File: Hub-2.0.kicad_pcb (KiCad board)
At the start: 2 copper layers, 120 x 78 mm, 9 parts, among them CN1 6437288-3, CN4 DT15-12PA, CN5 DT15-12PA, CN6 DT15-12PA, J3-PCB1 5569-06A2, U1 YQ506-S-112 DM

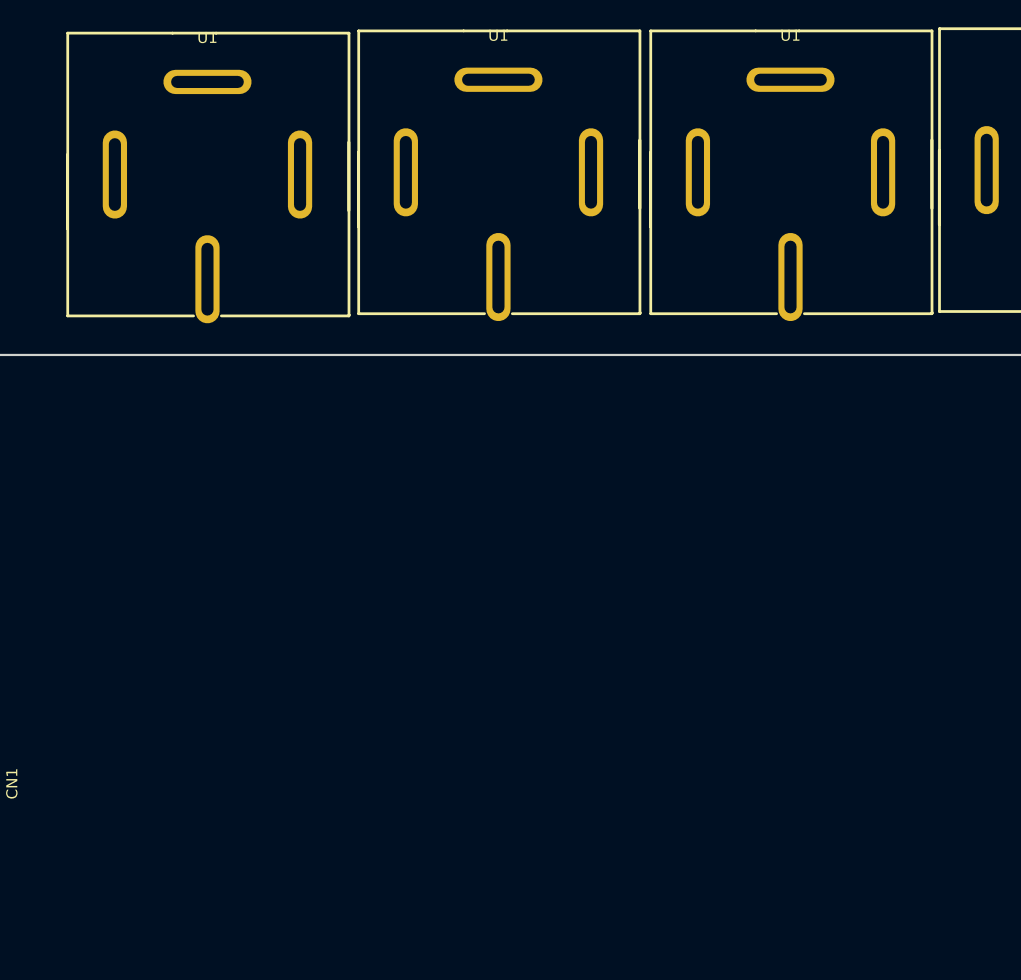
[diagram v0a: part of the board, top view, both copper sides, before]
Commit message: Autosave
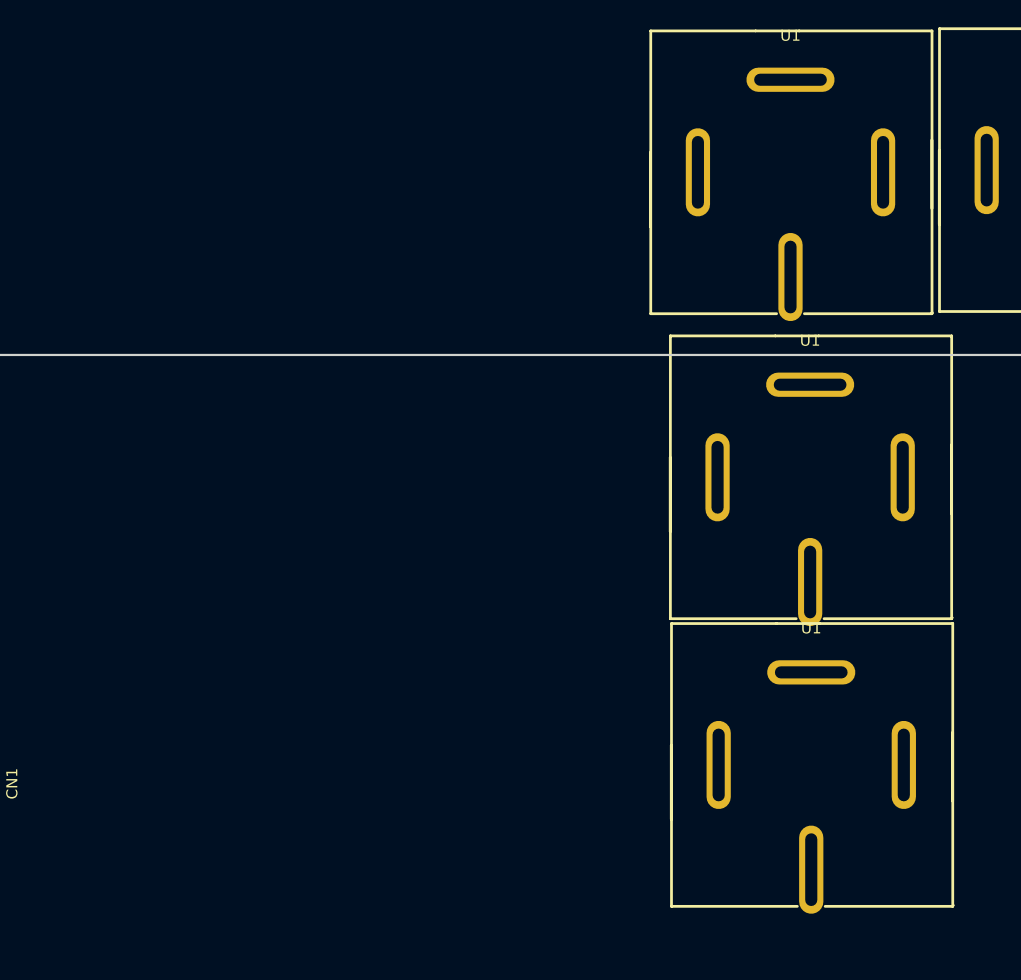
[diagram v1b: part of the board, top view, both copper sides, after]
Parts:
- moved U1 61.2 mm to (143.6, 40.5)
- moved U1 60.8 mm to (143.7, 66.5)
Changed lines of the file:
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@@
 	(footprint "EasyEDA:RELAY-TH_YQ506-S-112DM"
 		(layer "F.Cu")
-		(at 115.317502 12.7775)
+		(at 143.7 66.55)
 		(property "Reference" "U1"
 			(at 0 -12.95 0)
@@
 	(footprint "EasyEDA:RELAY-TH_YQ506-S-112DM"
 		(layer "F.Cu")
-		(at 88.9175 12.9775)
+		(at 143.6 40.45)
 		(property "Reference" "U1"
 			(at 0 -12.95 0)

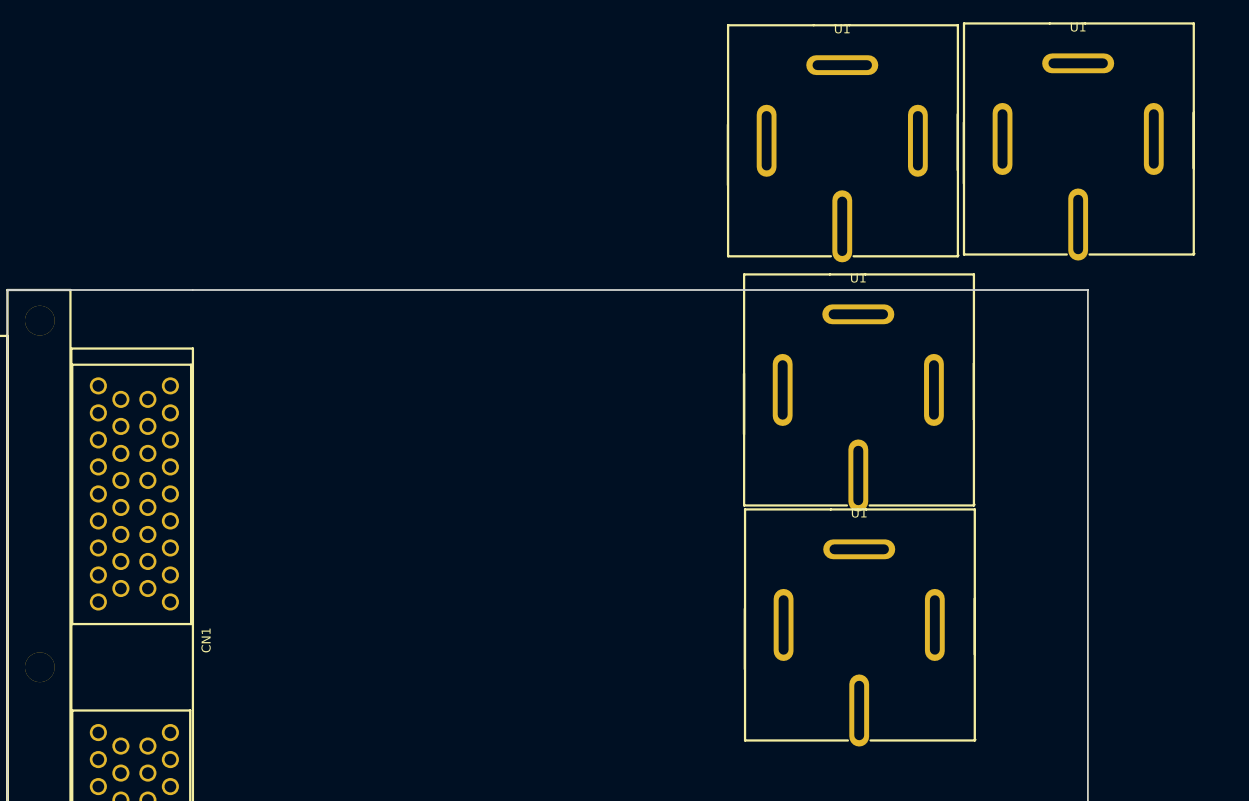
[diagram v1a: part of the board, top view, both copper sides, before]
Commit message: Autosave
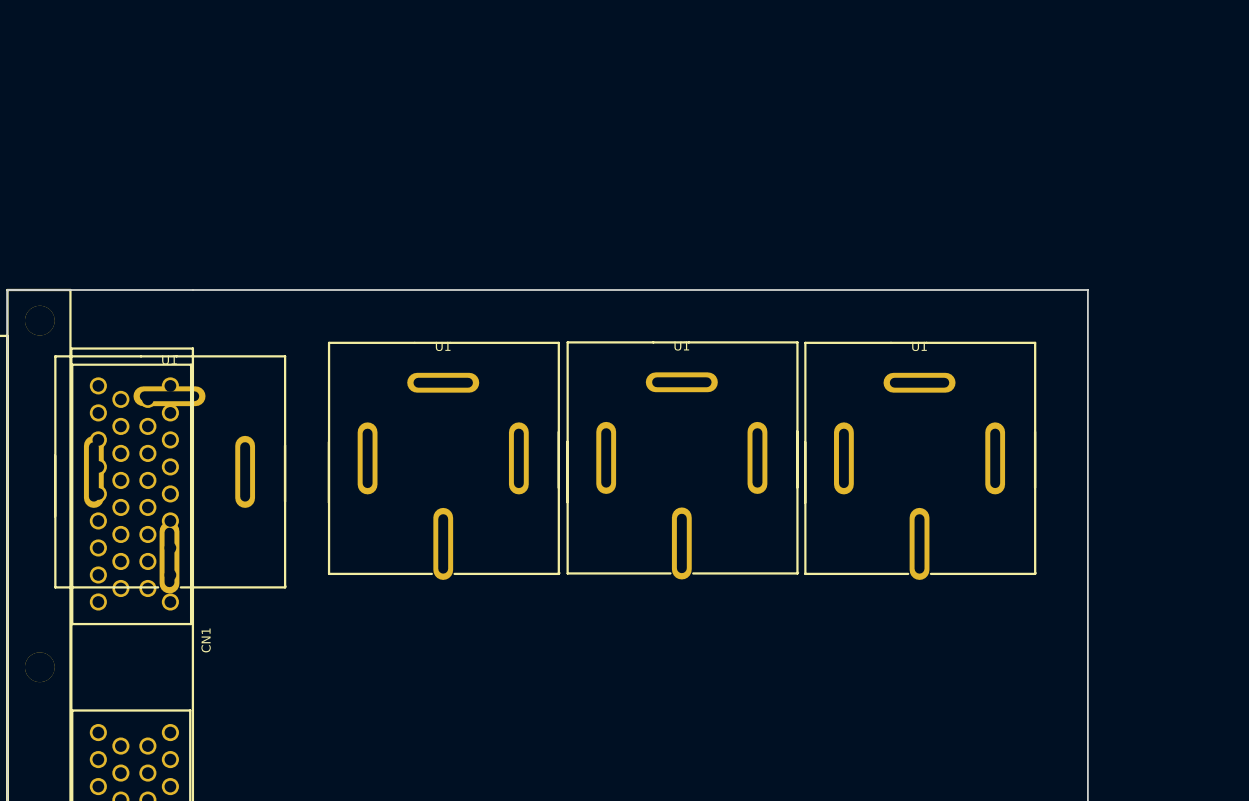
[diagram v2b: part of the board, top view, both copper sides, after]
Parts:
- moved U1 107.5 mm to (67.1, 49.5)
- moved U1 56.6 mm to (97.5, 48.0)
- moved U1 27.1 mm to (124.0, 48.0)
- moved U1 10.2 mm to (150.4, 48.0)
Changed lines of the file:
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@@
 	(footprint "EasyEDA:RELAY-TH_YQ506-S-112DM"
 		(layer "F.Cu")
-		(at 143.7 66.55)
+		(at 124 48)
 		(property "Reference" "U1"
 			(at 0 -12.95 0)
@@
 	(footprint "EasyEDA:RELAY-TH_YQ506-S-112DM"
 		(layer "F.Cu")
-		(at 143.6 40.45)
+		(at 150.4 48.05)
 		(property "Reference" "U1"
 			(at 0 -12.95 0)
@@
 	(footprint "EasyEDA:RELAY-TH_YQ506-S-112DM"
 		(layer "F.Cu")
-		(at 141.817501 12.7775)
+		(at 97.5 48.05)
 		(property "Reference" "U1"
 			(at 0 -12.95 0)
@@
 	(footprint "EasyEDA:RELAY-TH_YQ506-S-112DM"
 		(layer "F.Cu")
-		(at 168.0175 12.5775)
+		(at 67.1 49.55)
 		(property "Reference" "U1"
 			(at 0 -12.95 0)

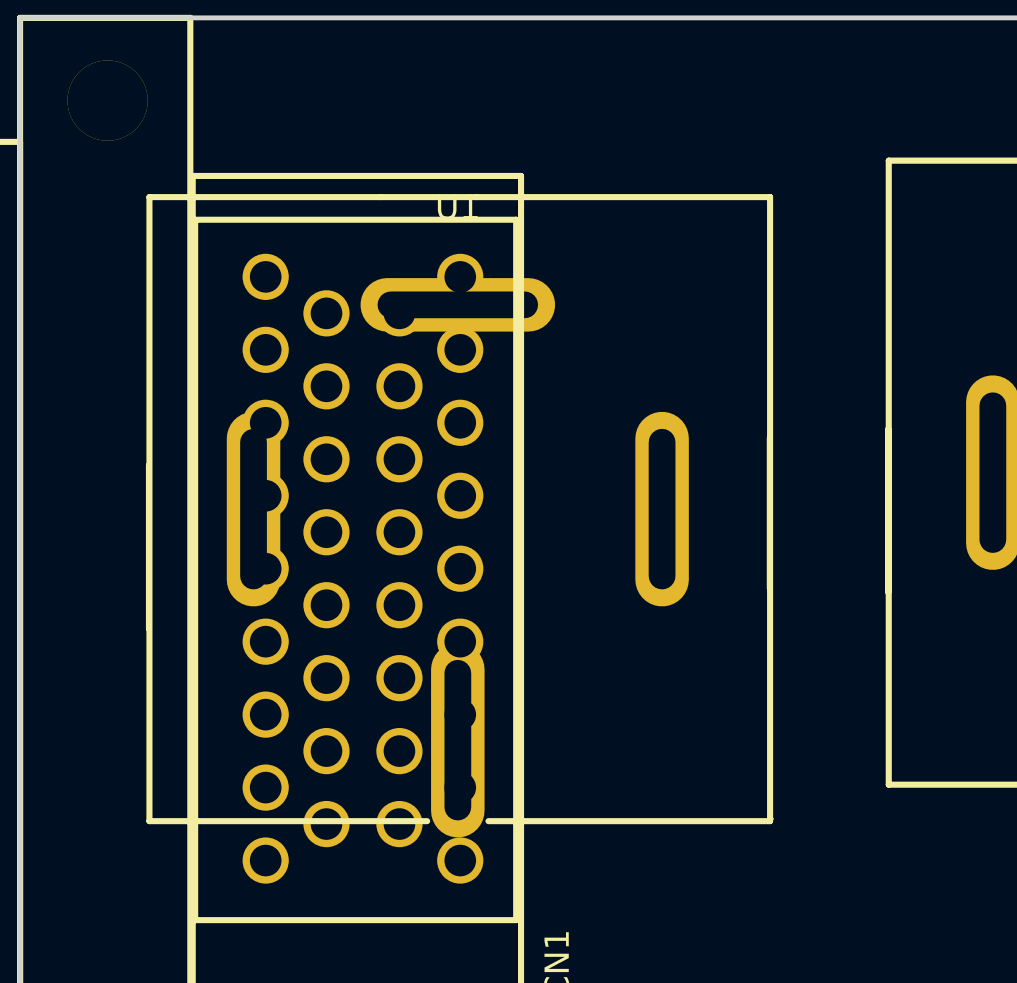
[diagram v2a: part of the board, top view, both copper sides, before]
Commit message: Autosave
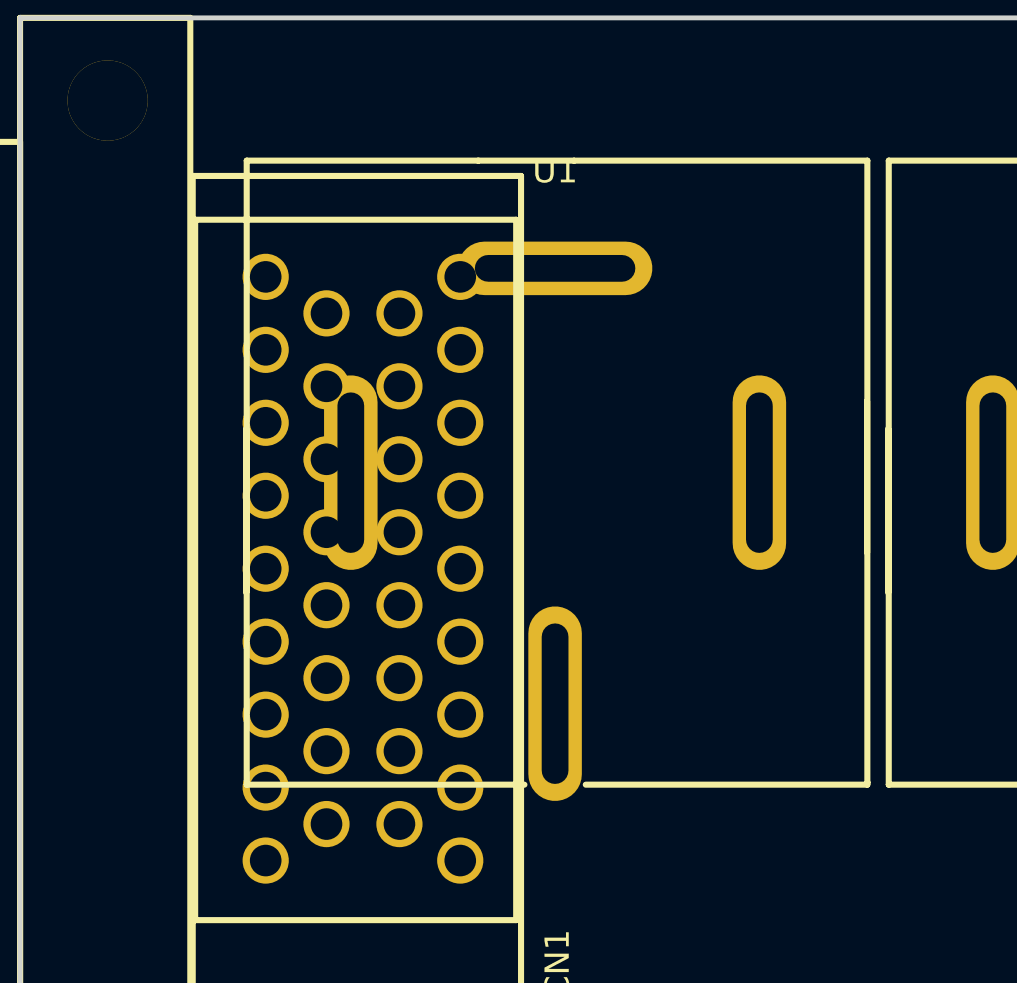
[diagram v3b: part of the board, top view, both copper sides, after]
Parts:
- moved U1 4.27 mm to (71.1, 48.0)
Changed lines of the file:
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@@
 	(footprint "EasyEDA:RELAY-TH_YQ506-S-112DM"
 		(layer "F.Cu")
-		(at 67.1 49.55)
+		(at 71.1 48.05)
 		(property "Reference" "U1"
 			(at 0 -12.95 0)

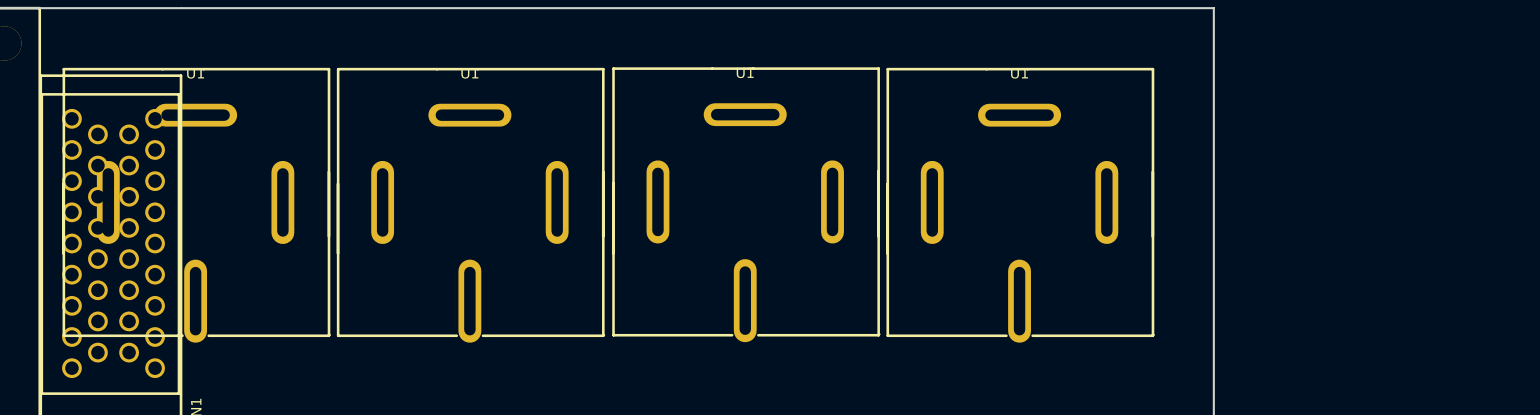
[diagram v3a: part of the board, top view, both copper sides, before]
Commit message: Autosave
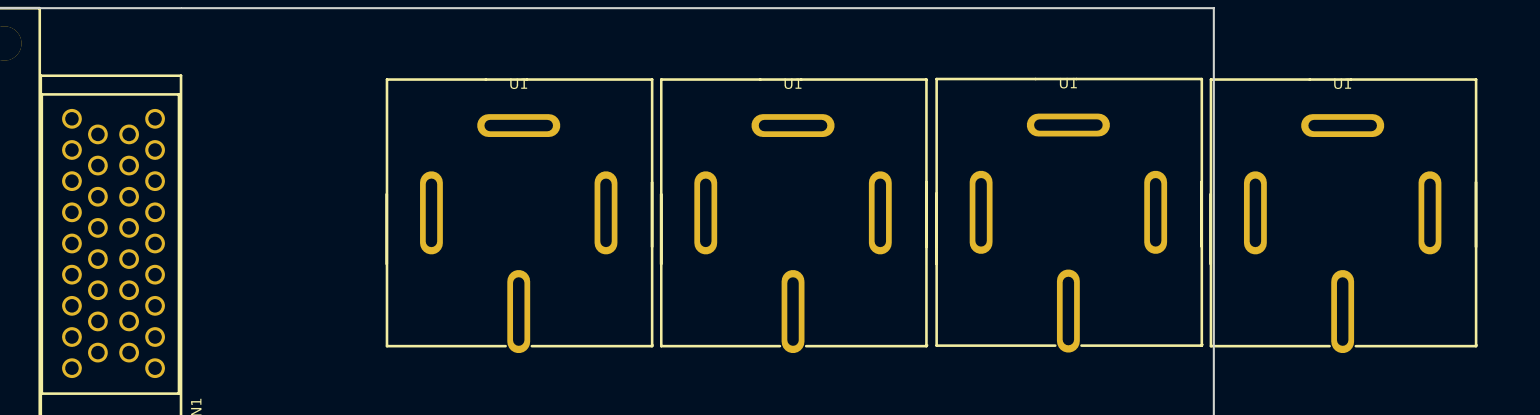
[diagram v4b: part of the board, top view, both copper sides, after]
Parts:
- moved U1 31.1 mm to (102.2, 49.0)
- moved U1 31.1 mm to (155.1, 49.0)
- moved U1 31.1 mm to (181.5, 49.0)
- moved U1 31.1 mm to (128.6, 49.0)
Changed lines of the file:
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@@
 	(footprint "EasyEDA:RELAY-TH_YQ506-S-112DM"
 		(layer "F.Cu")
-		(at 124 48)
+		(at 155.1 49)
 		(property "Reference" "U1"
 			(at 0 -12.95 0)
@@
 	(footprint "EasyEDA:RELAY-TH_YQ506-S-112DM"
 		(layer "F.Cu")
-		(at 150.4 48.05)
+		(at 181.5 49.05)
 		(property "Reference" "U1"
 			(at 0 -12.95 0)
@@
 	(footprint "EasyEDA:RELAY-TH_YQ506-S-112DM"
 		(layer "F.Cu")
-		(at 97.5 48.05)
+		(at 128.6 49.05)
 		(property "Reference" "U1"
 			(at 0 -12.95 0)
@@
 	(footprint "EasyEDA:RELAY-TH_YQ506-S-112DM"
 		(layer "F.Cu")
-		(at 71.1 48.05)
+		(at 102.2 49.05)
 		(property "Reference" "U1"
 			(at 0 -12.95 0)

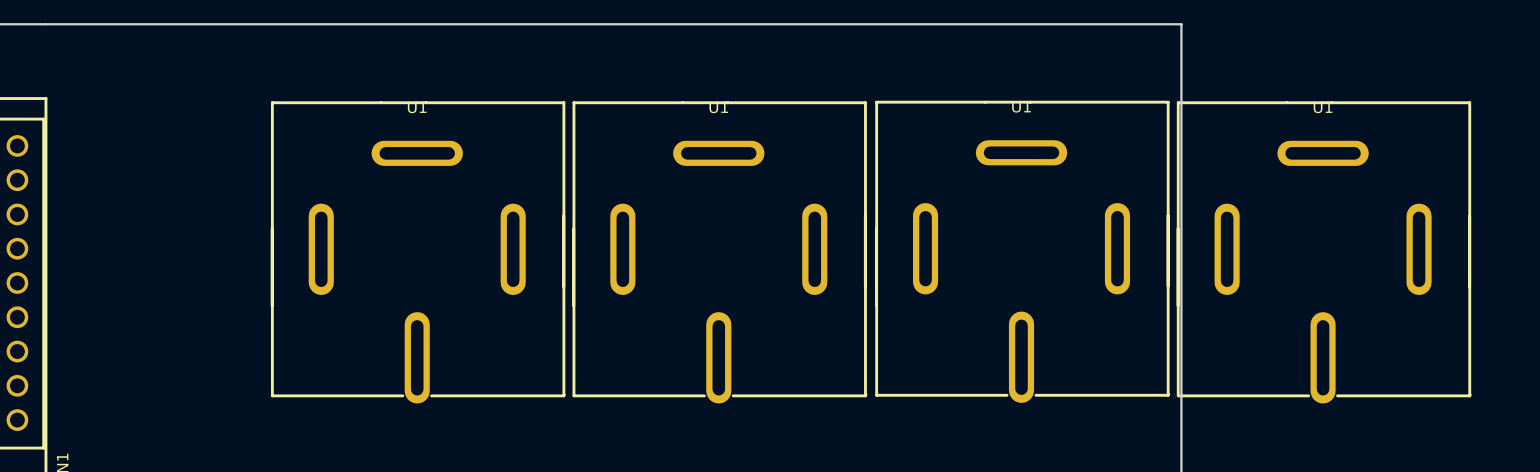
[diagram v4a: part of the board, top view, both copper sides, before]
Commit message: Autosave
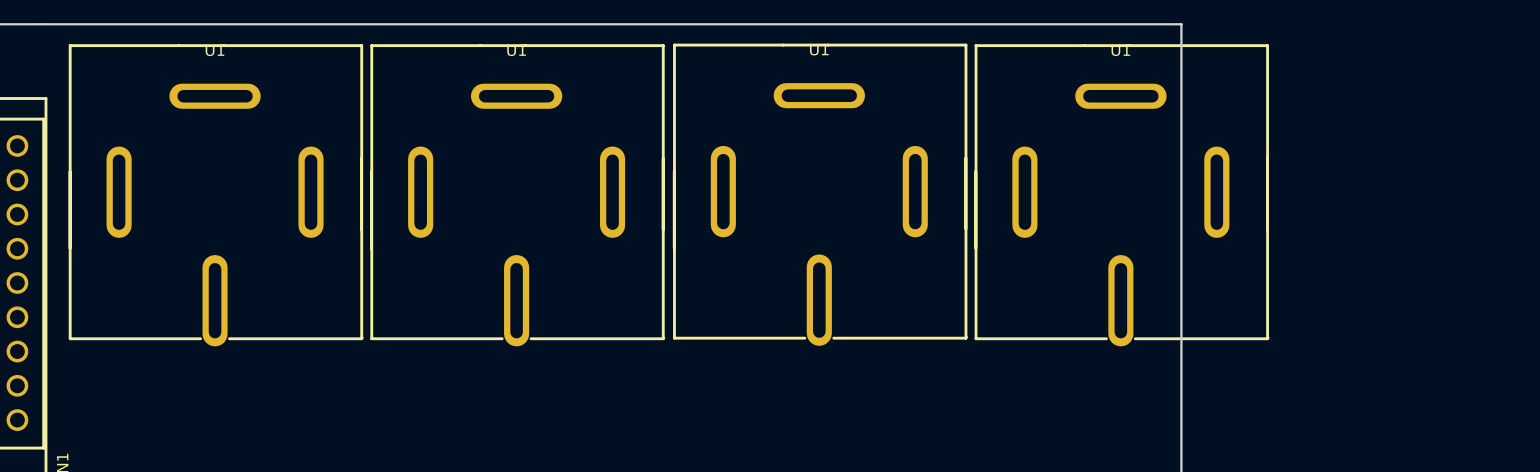
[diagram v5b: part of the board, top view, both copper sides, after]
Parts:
- moved U1 18.4 mm to (84.5, 44.0)
- moved U1 18.4 mm to (137.4, 44.0)
- moved U1 18.4 mm to (163.8, 44.0)
- moved U1 18.4 mm to (110.9, 44.0)
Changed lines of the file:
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@@
 	(footprint "EasyEDA:RELAY-TH_YQ506-S-112DM"
 		(layer "F.Cu")
-		(at 155.1 49)
+		(at 137.4 44)
 		(property "Reference" "U1"
 			(at 0 -12.95 0)
@@
 	(footprint "EasyEDA:RELAY-TH_YQ506-S-112DM"
 		(layer "F.Cu")
-		(at 181.5 49.05)
+		(at 163.8 44.05)
 		(property "Reference" "U1"
 			(at 0 -12.95 0)
@@
 	(footprint "EasyEDA:RELAY-TH_YQ506-S-112DM"
 		(layer "F.Cu")
-		(at 128.6 49.05)
+		(at 110.9 44.05)
 		(property "Reference" "U1"
 			(at 0 -12.95 0)
@@
 	(footprint "EasyEDA:RELAY-TH_YQ506-S-112DM"
 		(layer "F.Cu")
-		(at 102.2 49.05)
+		(at 84.5 44.05)
 		(property "Reference" "U1"
 			(at 0 -12.95 0)
